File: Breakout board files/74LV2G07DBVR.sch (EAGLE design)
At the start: 7 parts, among them IC1 SN74LVC2G07DBVR

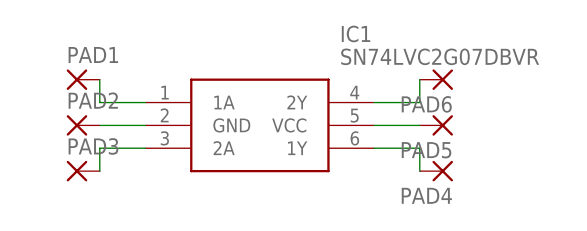
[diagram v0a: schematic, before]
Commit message: Breakout Board Solutions
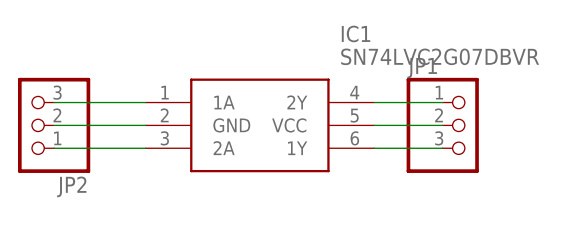
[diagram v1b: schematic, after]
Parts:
- removed PAD1, PAD2, PAD3, PAD4, PAD5, PAD6: (no value), ee2parts:PAD-TERMINAL
- added JP1, JP2: (no value), pinhead:PINHD-1X3
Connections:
- net N$1: now also JP2.2; no longer PAD2.P
- net N$2: now also JP2.3; no longer PAD1.P
- net N$3: now also JP2.1; no longer PAD3.P
- net N$4: now also JP1.3; no longer PAD4.P
- net N$5: now also JP1.1; no longer PAD6.P
- net N$6: now also JP1.2; no longer PAD5.P
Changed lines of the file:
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@@
 <?xml version="1.0" encoding="utf-8"?>
 <!DOCTYPE eagle SYSTEM "eagle.dtd">
-<eagle version="8.3.2">
+<eagle version="9.2.0">
 <drawing>
 <settings>
@@
 <layers>
 <layer number="1" name="Top" color="4" fill="1" visible="no" active="no"/>
+<layer number="2" name="Route2" color="1" fill="3" visible="no" active="no"/>
+<layer number="3" name="Route3" color="4" fill="3" visible="no" active="no"/>
+<layer number="4" name="Route4" color="1" fill="4" visible="no" active="no"/>
+<layer number="5" name="Route5" color="4" fill="4" visible="no" active="no"/>
+<layer number="6" name="Route6" color="1" fill="8" visible="no" active="no"/>
+<layer number="7" name="Route7" color="4" fill="8" visible="no" active="no"/>
+<layer number="8" name="Route8" color="1" fill="2" visible="no" active="no"/>
+<layer number="9" name="Route9" color="4" fill="2" visible="no" active="no"/>
+<layer number="10" name="Route10" color="1" fill="7" visible="no" active="no"/>
+<layer number="11" name="Route11" color="4" fill="7" visible="no" active="no"/>
+<layer number="12" name="Route12" color="1" fill="5" visible="no" active="no"/>
+<layer number="13" name="Route13" color="4" fill="5" visible="no" active="no"/>
+<layer number="14" name="Route14" color="1" fill="6" visible="no" active="no"/>
+<layer number="15" name="Route15" color="4" fill="6" visible="no" active="no"/>
 <layer number="16" name="Bottom" color="1" fill="1" visible="no" active="no"/>
 <layer number="17" name="Pads" color="2" fill="1" visible="no" active="no"/>
@@
 <parts>
 <part name="IC1" library="SN74LVC2G07DBVR" deviceset="SN74LVC2G07DBVR" device=""/>
-<part name="PAD1" library="ee2parts" deviceset="PAD-TERMINAL" device=""/>
-<part name="PAD2" library="ee2parts" deviceset="PAD-TERMINAL" device=""/>
-<part name="PAD3" library="ee2parts" deviceset="PAD-TERMINAL" device=""/>
-<part name="PAD4" library="ee2parts" deviceset="PAD-TERMINAL" device=""/>
-<part name="PAD5" library="ee2parts" deviceset="PAD-TERMINAL" device=""/>
-<part name="PAD6" library="ee2parts" deviceset="PAD-TERMINAL" device=""/>
+<part name="JP1" library="pinhead" library_urn="urn:adsk.eagle:library:325" deviceset="PINHD-1X3" device="" package3d_urn="urn:adsk.eagle:package:22458/2"/>
+<part name="JP2" library="pinhead" library_urn="urn:adsk.eagle:library:325" deviceset="PINHD-1X3" device="" package3d_urn="urn:adsk.eagle:package:22458/2"/>
 </parts>
 <sheets>
@@
 </plain>
 <instances>
-<instance part="IC1" gate="G$1" x="63.5" y="45.72"/>
-<instance part="PAD1" gate="1" x="55.88" y="48.26"/>
-<instance part="PAD2" gate="1" x="55.88" y="43.18"/>
-<instance part="PAD3" gate="1" x="55.88" y="38.1"/>
-<instance part="PAD4" gate="1" x="96.52" y="38.1" rot="R180"/>
-<instance part="PAD5" gate="1" x="96.52" y="43.18" rot="R180"/>
-<instance part="PAD6" gate="1" x="96.52" y="48.26" rot="R180"/>
+<instance part="IC1" gate="G$1" x="63.5" y="45.72">
+<attribute name="NAME" x="85.09" y="53.34" size="1.778" layer="95" align="center-left"/>
+<attribute name="VALUE" x="85.09" y="50.8" size="1.778" layer="96" align="center-left"/>
+</instance>
+<instance part="JP1" gate="A" x="99.06" y="43.18">
+<attribute name="NAME" x="92.71" y="48.895" size="1.778" layer="95"/>
+<attribute name="VALUE" x="92.71" y="35.56" size="1.778" layer="96"/>
+</instance>
+<instance part="JP2" gate="A" x="50.8" y="43.18" rot="R180">
+<attribute name="NAME" x="57.15" y="37.465" size="1.778" layer="95" rot="R180"/>
+<attribute name="VALUE" x="57.15" y="50.8" size="1.778" layer="96" rot="R180"/>
+</instance>
 </instances>
 <busses>
@@
 <segment>
 <pinref part="IC1" gate="G$1" pin="GND"/>
-<pinref part="PAD2" gate="1" pin="P"/>
-<wire x1="63.5" y1="43.18" x2="58.42" y2="43.18" width="0.1524" layer="91"/>
+<pinref part="JP2" gate="A" pin="2"/>
+<wire x1="63.5" y1="43.18" x2="53.34" y2="43.18" width="0.1524" layer="91"/>
 </segment>
 </net>
@@
 <segment>
 <pinref part="IC1" gate="G$1" pin="1A"/>
-<pinref part="PAD1" gate="1" pin="P"/>
-<wire x1="63.5" y1="45.72" x2="58.42" y2="45.72" width="0.1524" layer="91"/>
-<wire x1="58.42" y1="45.72" x2="58.42" y2="48.26" width="0.1524" layer="91"/>
+<pinref part="JP2" gate="A" pin="3"/>
+<wire x1="63.5" y1="45.72" x2="53.34" y2="45.72" width="0.1524" layer="91"/>
 </segment>
 </net>
 <net name="N$3" class="0">
 <segment>
-<pinref part="PAD3" gate="1" pin="P"/>
-<wire x1="58.42" y1="38.1" x2="58.42" y2="40.64" width="0.1524" layer="91"/>
 <pinref part="IC1" gate="G$1" pin="2A"/>
-<wire x1="58.42" y1="40.64" x2="63.5" y2="40.64" width="0.1524" layer="91"/>
+<pinref part="JP2" gate="A" pin="1"/>
+<wire x1="63.5" y1="40.64" x2="53.34" y2="40.64" width="0.1524" layer="91"/>
 </segment>
 </net>
@@
 <segment>
 <pinref part="IC1" gate="G$1" pin="1Y"/>
-<pinref part="PAD4" gate="1" pin="P"/>
-<wire x1="88.9" y1="40.64" x2="93.98" y2="40.64" width="0.1524" layer="91"/>
-<wire x1="93.98" y1="40.64" x2="93.98" y2="38.1" width="0.1524" layer="91"/>
+<wire x1="88.9" y1="40.64" x2="96.52" y2="40.64" width="0.1524" layer="91"/>
+<pinref part="JP1" gate="A" pin="3"/>
 </segment>
 </net>
 <net name="N$5" class="0">
 <segment>
-<pinref part="PAD6" gate="1" pin="P"/>
-<wire x1="93.98" y1="48.26" x2="93.98" y2="45.72" width="0.1524" layer="91"/>
 <pinref part="IC1" gate="G$1" pin="2Y"/>
-<wire x1="93.98" y1="45.72" x2="88.9" y2="45.72" width="0.1524" layer="91"/>
+<wire x1="96.52" y1="45.72" x2="88.9" y2="45.72" width="0.1524" layer="91"/>
+<pinref part="JP1" gate="A" pin="1"/>
 </segment>
 </net>
@@
 <segment>
 <pinref part="IC1" gate="G$1" pin="VCC"/>
-<pinref part="PAD5" gate="1" pin="P"/>
-<wire x1="88.9" y1="43.18" x2="93.98" y2="43.18" width="0.1524" layer="91"/>
+<wire x1="88.9" y1="43.18" x2="96.52" y2="43.18" width="0.1524" layer="91"/>
+<pinref part="JP1" gate="A" pin="2"/>
 </segment>
 </net>
@@
 </schematic>
 </drawing>
+<compatibility>
+<note version="8.2" severity="warning">
+Since Version 8.2, EAGLE supports online libraries. The ids
+of those online libraries will not be understood (or retained)
+with this version.
+</note>
+<note version="8.3" severity="warning">
+Since Version 8.3, EAGLE supports URNs for individual library
+assets (packages, symbols, and devices). The URNs of those assets
+will not be understood (or retained) with this version.
+</note>
+<note version="8.3" severity="warning">
+Since Version 8.3, EAGLE supports the association of 3D packages
+with devices in libraries, schematics, and board files. Those 3D
+packages will not be understood (or retained) with this version.
+</note>
+</compatibility>
 </eagle>
